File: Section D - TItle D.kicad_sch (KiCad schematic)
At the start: 11 parts, among them Q2 CSD18534Q5A, Q3 BSS123, Q4 BSS84, Q5 BSS123

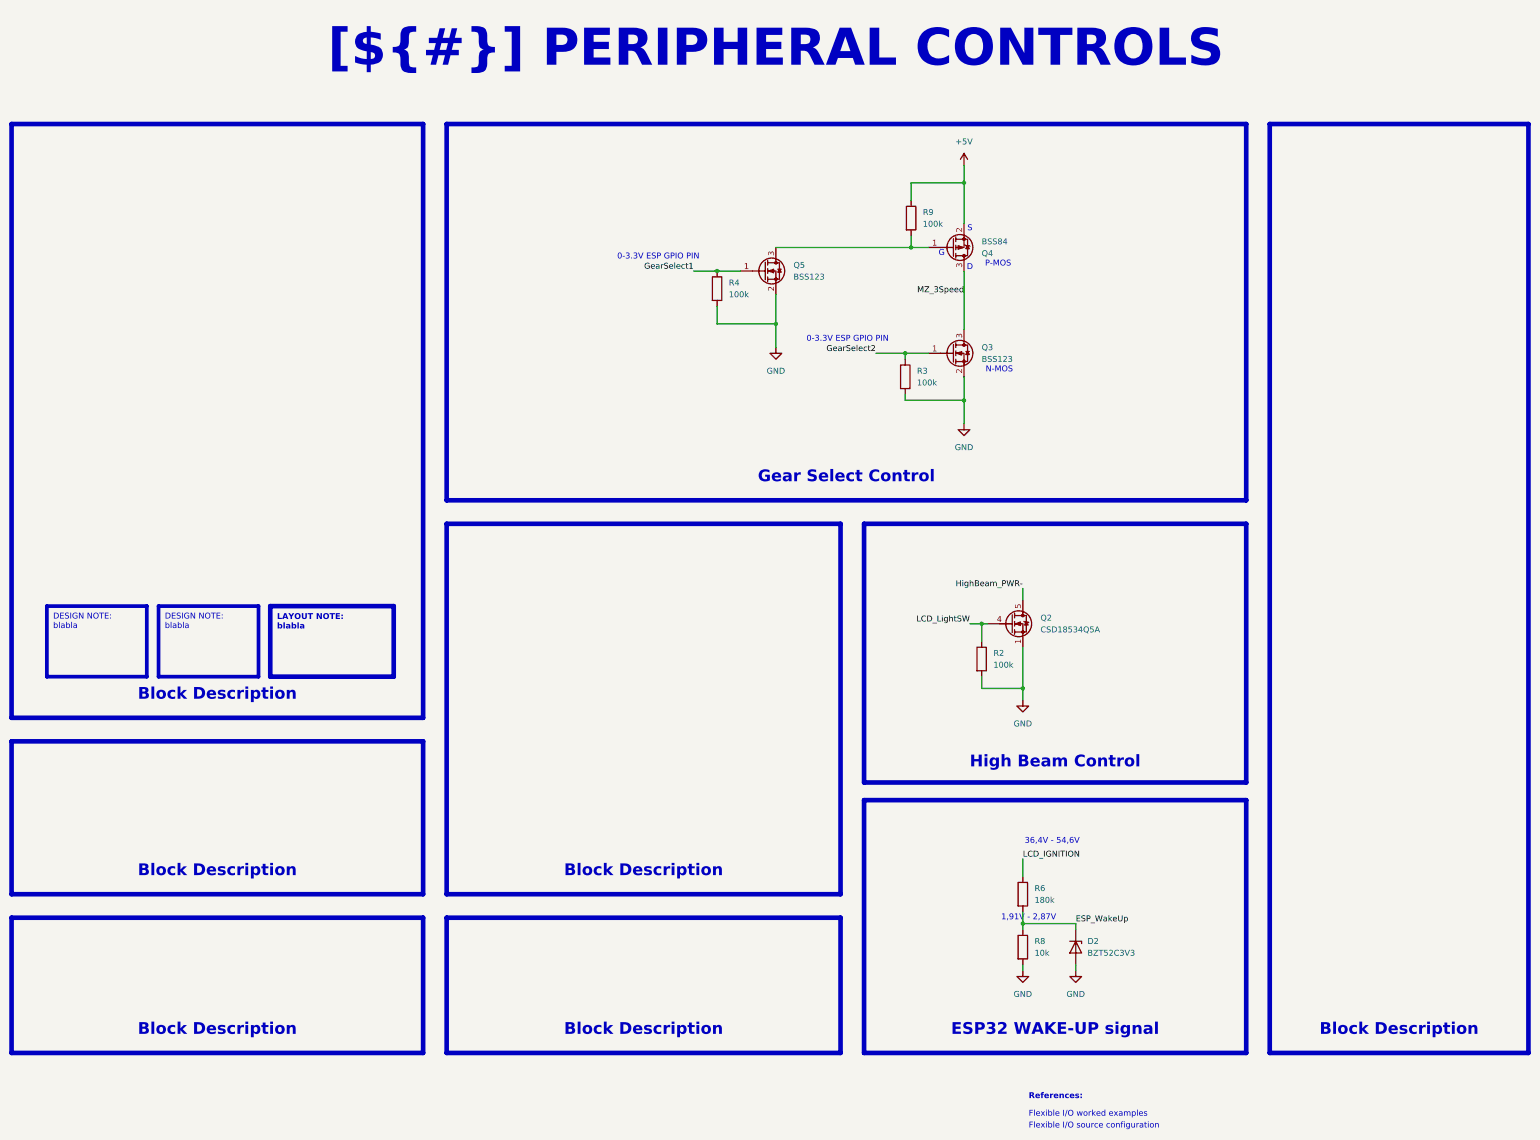
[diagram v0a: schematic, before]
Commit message: 1st PCB prototype traced
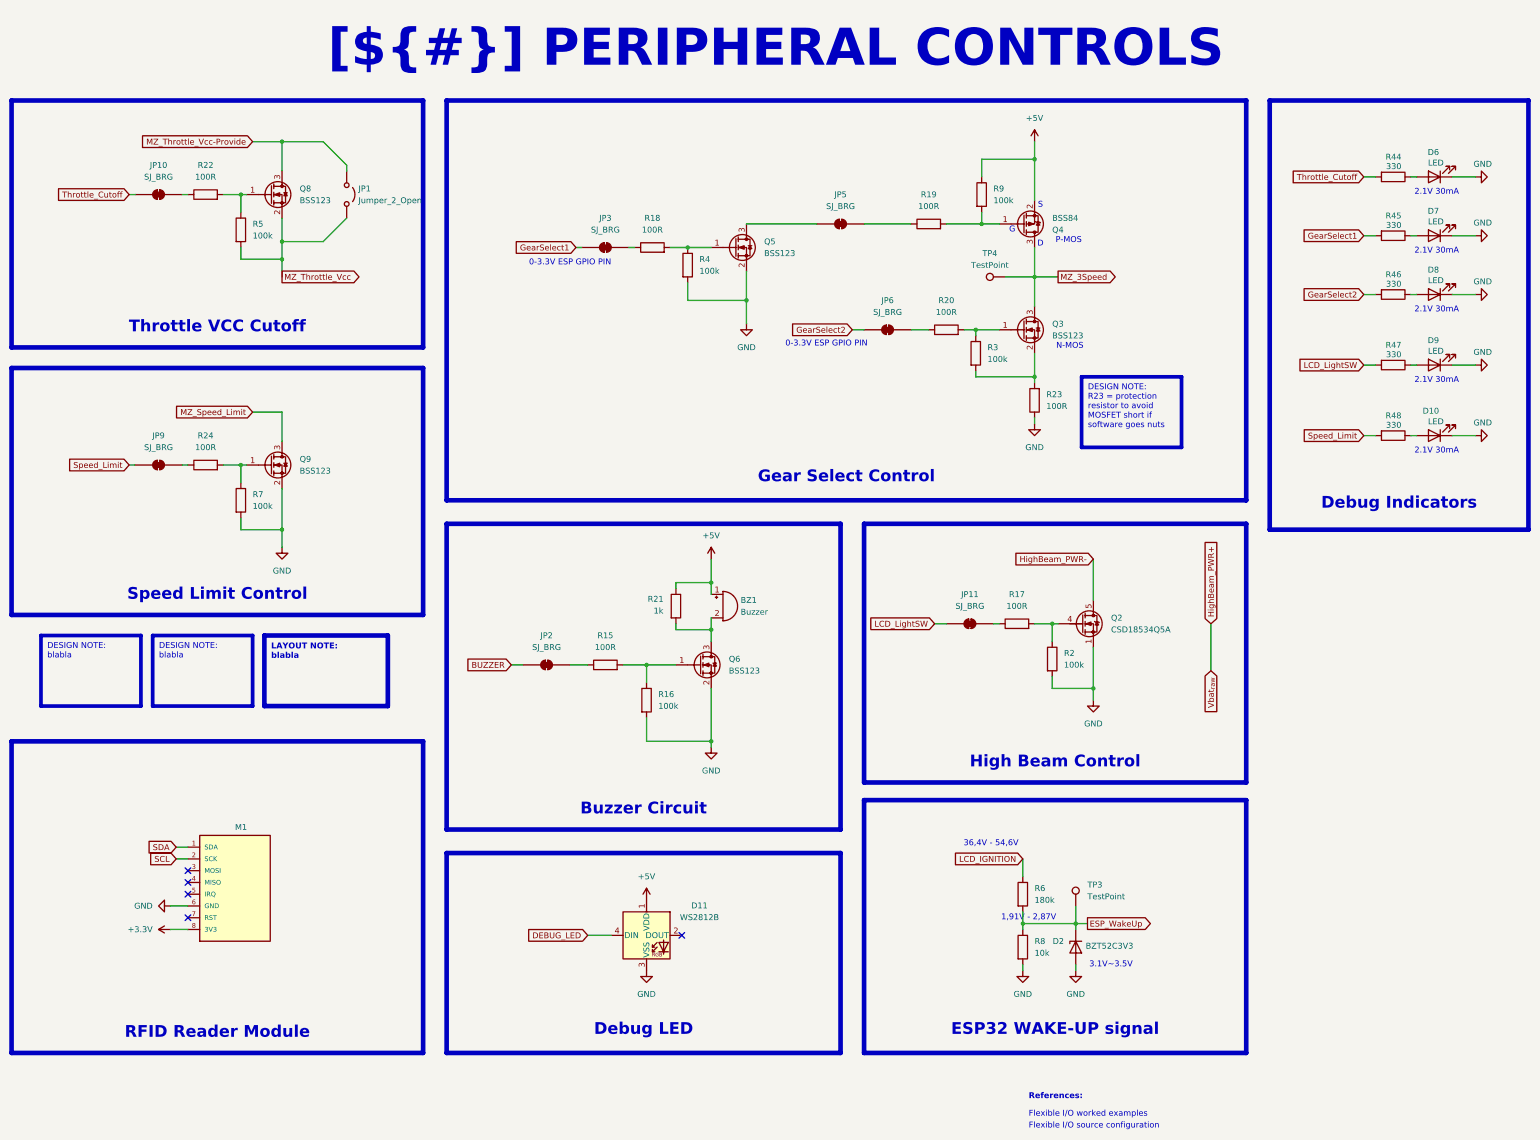
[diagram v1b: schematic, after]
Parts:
- added BZ1: Buzzer, Buzzer_Beeper:MagneticBuzzer_PUI_AT-0927-TT-6-R, symbol Device:Buzzer
- added D10, D6, D7, D8, D9: LED, LED_SMD:LED_0603_1608Metric, symbol Device:LED
- added D11: WS2812B, LED_SMD:LED_WS2812B_PLCC4_5.0x5.0mm_P3.2mm, symbol LED:WS2812B
- added JP1: Jumper_2_Open, Jumper:SolderJumper-2_P1.3mm_Open_Pad1.0x1.5mm, symbol Jumper:Jumper_2_Open
- added JP10, JP11, JP2, JP3, JP5, JP6, JP9: SJ_BRG, Jumper:SolderJumper-2_P1.3mm_Bridged_Pad1.0x1.5mm, symbol Jumper:SolderJumper_2_Bridged
- added M1: (no value), BRADES_Modules:RFID-RC522, symbol BRADES_Modules:RFID-RC522
- added Q6, Q8, Q9: BSS123, Package_TO_SOT_SMD:SOT-23, symbol Transistor_FET:BSS123
- added R15, R17, R18, R19, R20, R22, R23, R24: 100R, Resistor_SMD:R_0603_1608Metric_Pad0.98x0.95mm_HandSolder, symbol Device:R
- added R16, R5, R7: 100k, Resistor_SMD:R_0603_1608Metric_Pad0.98x0.95mm_HandSolder, symbol Device:R
- added R21: 1k, Resistor_SMD:R_0603_1608Metric_Pad0.98x0.95mm_HandSolder, symbol Device:R
- added R44, R45, R46, R47, R48: 330, Resistor_SMD:R_0603_1608Metric, symbol Device:R
- added TP3, TP4: TestPoint, TestPoint:TestPoint_Pad_1.5x1.5mm, symbol Connector:TestPoint
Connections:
- net +5V: now also BZ1.1 (+), D11.1 (VDD), R21.1
- net ESP_WakeUp: now also TP3.1
- net GND: now also D10.1 (K), D11.3 (VSS), D6.1 (K), D7.1 (K), D8.1 (K), D9.1 (K), M1.6 (GND), Q6.2 (S), Q9.2 (S), R16.2, R23.1, R7.2; no longer Q3.2 (S), R3.2
- net GearSelect1: now also JP3.1 (A), R45.2; no longer Q5.1 (G), R4.1
- net GearSelect2: now also JP6.1 (A), R46.2; no longer Q3.1 (G), R3.1
- net LCD_LightSW: now also JP11.1 (A), R47.2; no longer Q2.4 (G), R2.1
- net MZ_3Speed: now also TP4.1
- net at Q4.1 (G), R9.2: now also R19.2; no longer Q5.3 (D)
- new net: JP2.2 (B), R15.1
- new net: Q6.1 (G), R15.2, R16.1
- new net: Q3.1 (G), R20.2, R3.1
- new net: Q3.2 (S), R23.2, R3.2
- new net: D8.2 (A), R46.1
- new net: JP11.2 (B), R17.1
- new net: Q8.1 (G), R22.2, R5.1
- new net: BZ1.2 (-), Q6.3 (D), R21.2
- new net: JP10.2 (B), R22.1
- new net: Q2.4 (G), R17.2, R2.1
- new net: JP9.2 (B), R24.1
- new net: Q9.1 (G), R24.2, R7.1
- new net: D7.2 (A), R45.1
- new net: D9.2 (A), R47.1
- new net: D10.2 (A), R48.1
- new net: JP6.2 (B), R20.1
- new net: JP3.2 (B), R18.1
- new net: Q5.1 (G), R18.2, R4.1
- new net: JP5.1 (A), Q5.3 (D)
- new net: JP5.2 (B), R19.1
- new net: D6.2 (A), R44.1
- new net +3.3V: M1.8 (3V3)
- new net BUZZER: JP2.1 (A)
- new net DEBUG_LED: D11.4 (DIN)
- new net MZ_Speed_Limit: Q9.3 (D)
- new net MZ_Throttle_Vcc: JP1.2 (B), Q8.2 (S), R5.2
- new net MZ_Throttle_Vcc-Provide: JP1.1 (A), Q8.3 (D)
- new net SCL: M1.2 (SCK)
- new net SDA: M1.1 (SDA)
- new net Speed_Limit: JP9.1 (A), R48.2
- new net Throttle_Cutoff: JP10.1 (A), R44.2
- no-connect marks 0 -> 5
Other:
- note added: "2.1V 30mA"
- note added: "3.1V~3.5V"
- moved on the sheet: D2, Q2, Q3, Q4, Q5, R2, R3, R4, R9
